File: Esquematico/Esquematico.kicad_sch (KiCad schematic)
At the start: 15 parts, among them SW1 Pulsador, SW2 Pulsador, U1 ATmega328P-P, U2 L7805, Y1 16Mhz

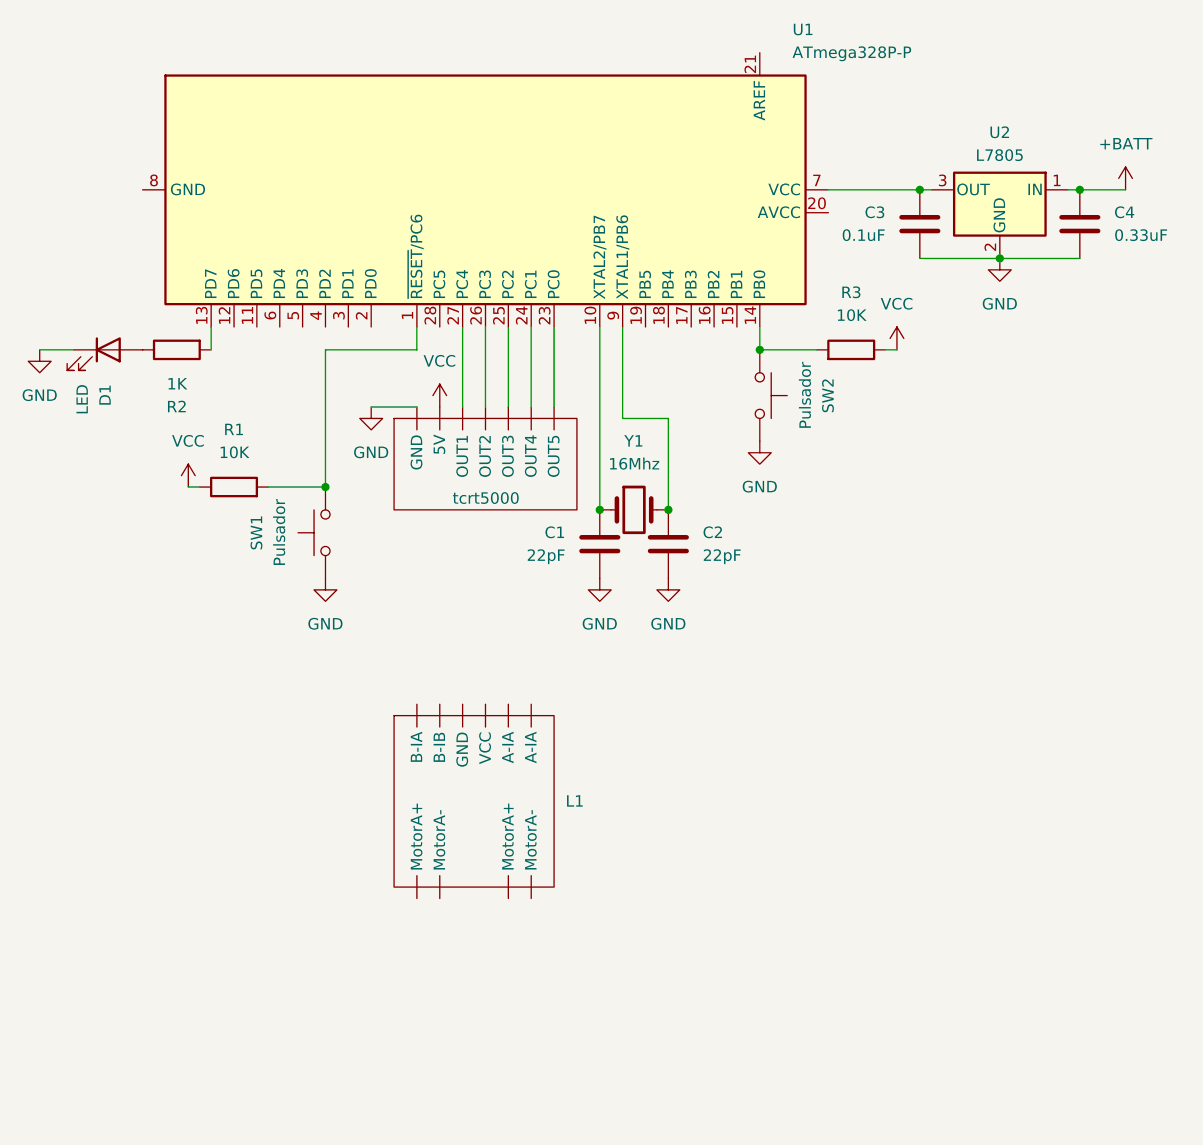
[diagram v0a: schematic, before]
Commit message: Termino el esquemático
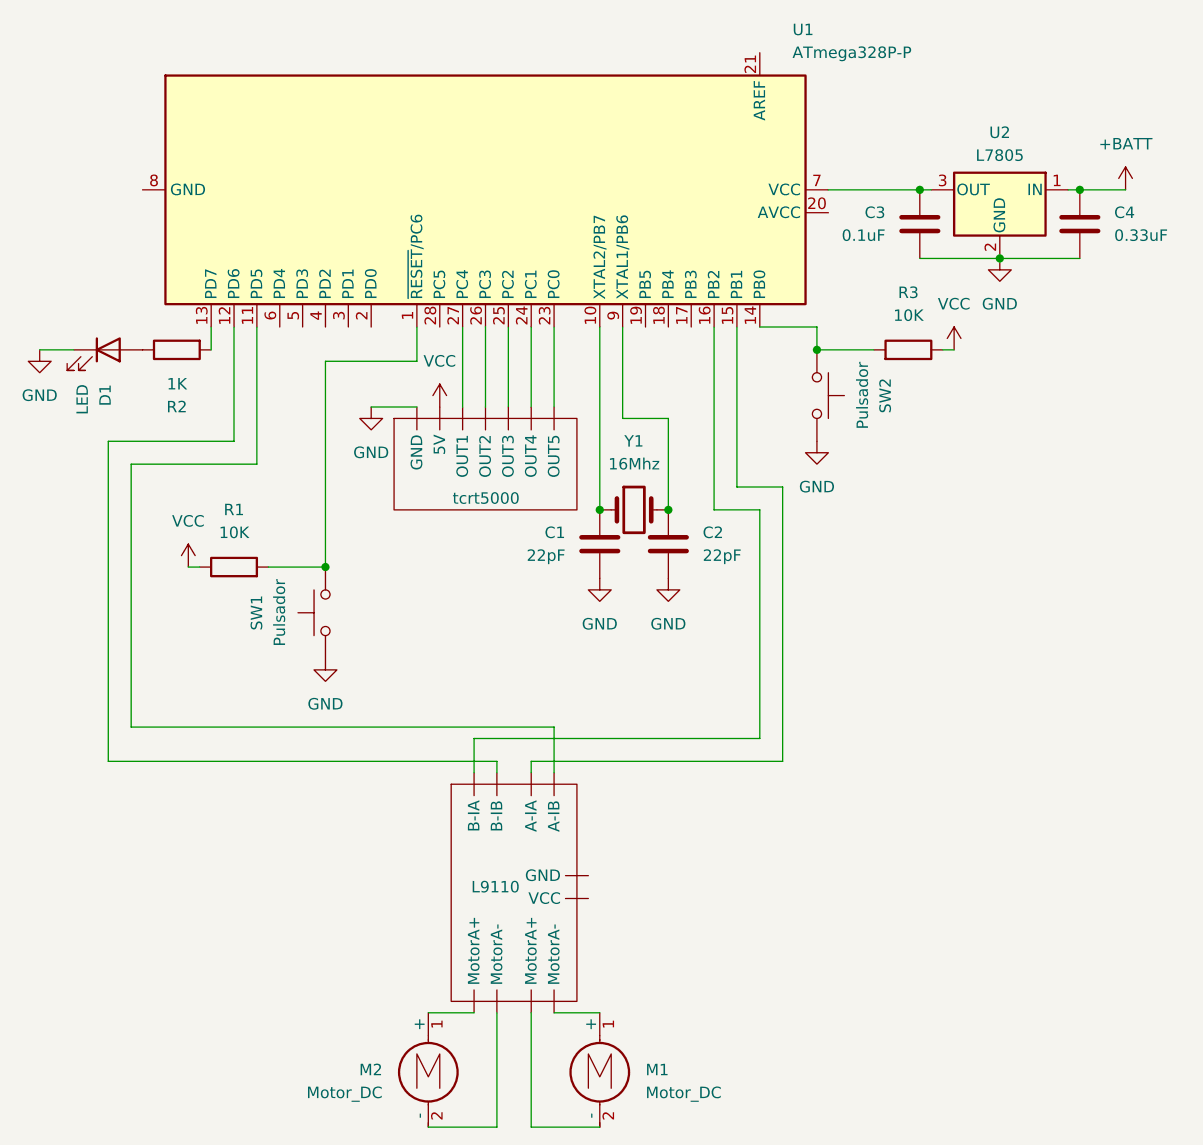
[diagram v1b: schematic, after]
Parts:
- removed L1: ~, symbol L9110:L9110
- added L9110: ~, symbol L9110:L9110
- added M1, M2: Motor_DC, symbol Motor:Motor_DC
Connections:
- net at U1.11 (PD5): now also L9110. (VCC)
- net at U1.12 (PD6): now also L9110. (VCC)
- net at U1.15 (PB1): now also L9110. (VCC)
- net at U1.16 (PB2): now also L9110. (VCC)
- new net: L9110. (VCC), M1.1 (+)
- new net: L9110. (VCC), M1.2 (-)
- new net: L9110. (VCC), M2.1 (+)
- new net: L9110. (VCC), M2.2 (-)
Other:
- moved on the sheet: R1, R3, SW1, SW2
